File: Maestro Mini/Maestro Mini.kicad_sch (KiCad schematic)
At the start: 13 parts, among them SW1 SW_Push, SW10 SW_Push, SW2 SW_Push, SW3 SW_Push, SW4 SW_Push, SW5 SW_Push, SW6 SW_Push, SW7 SW_Push, SW8 SW_Push, SW9 SW_Push, U1 MCP23017x-x-SP

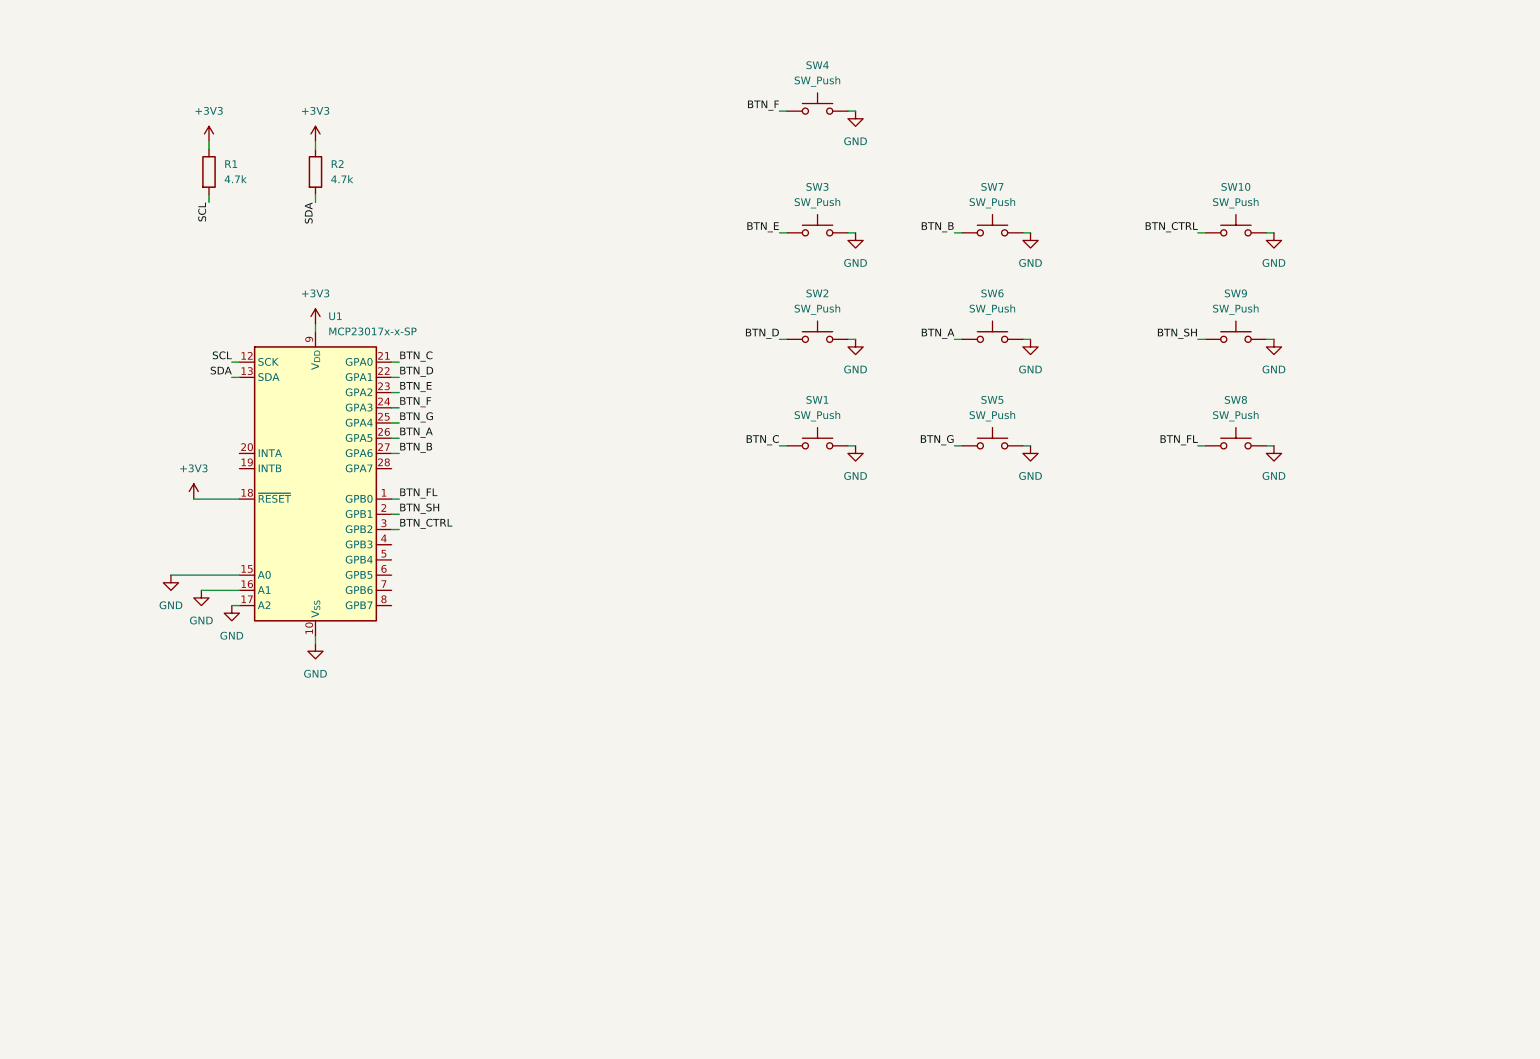
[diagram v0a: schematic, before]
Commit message: Finalized the schematics.
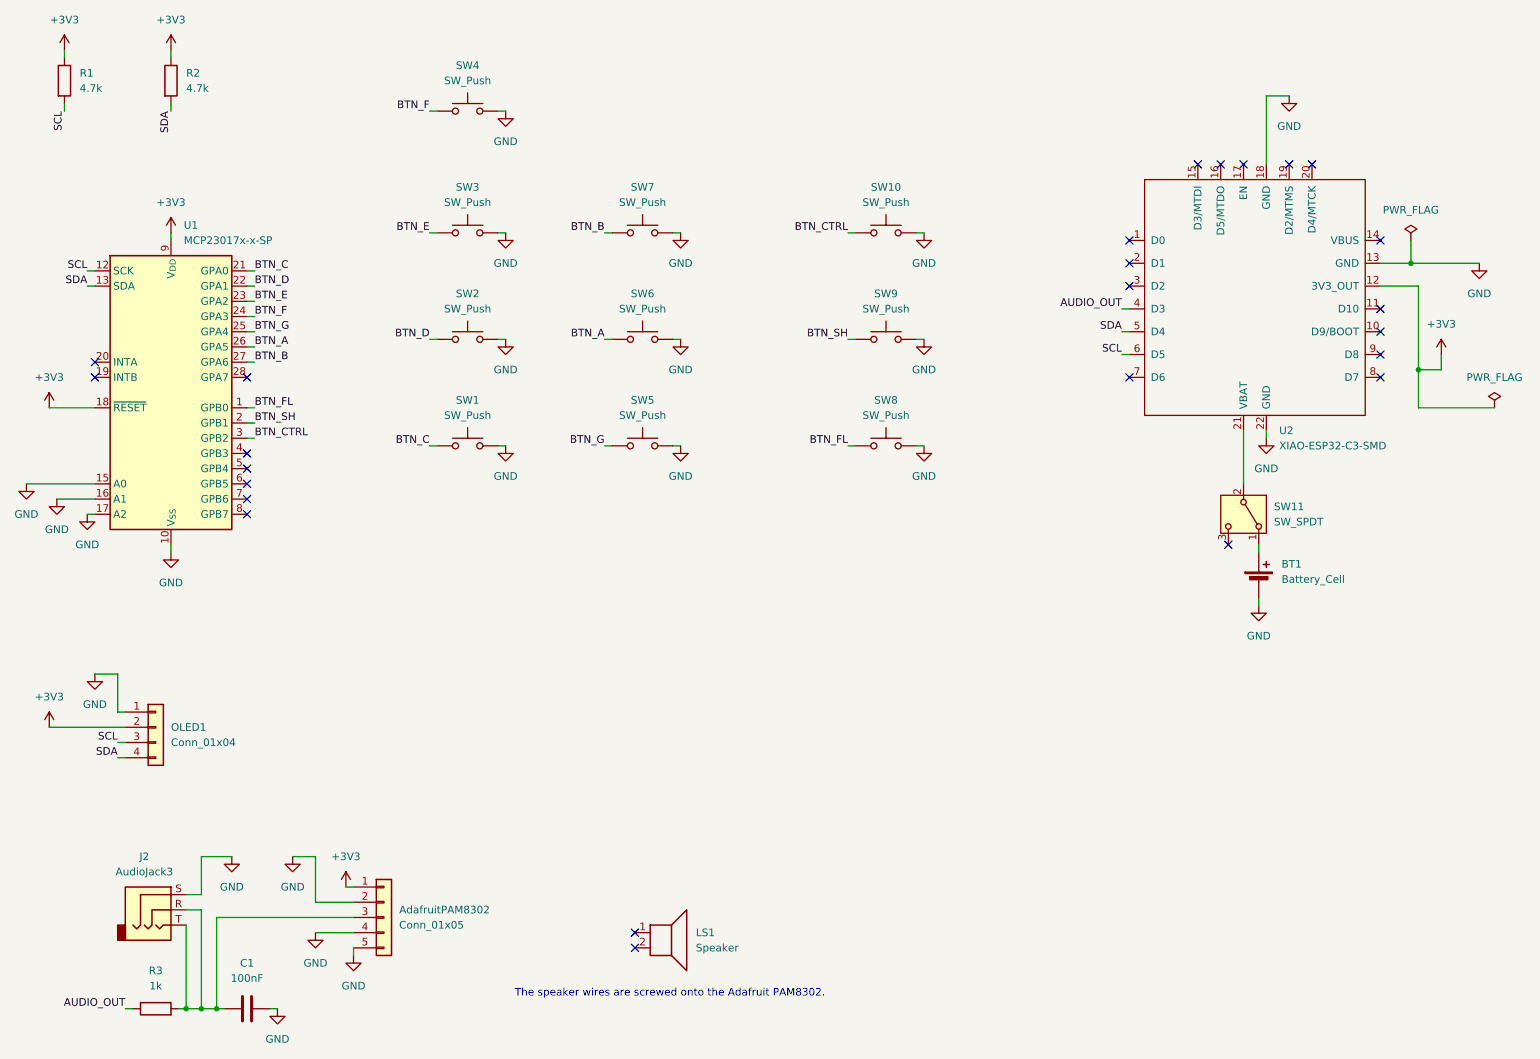
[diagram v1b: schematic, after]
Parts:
- added AdafruitPAM8302: Conn_01x05, symbol Connector_Generic:Conn_01x05
- added BT1: Battery_Cell, Package_DFN_QFN:QFN-40-1EP_6x6mm_P0.5mm_EP4.6x4.6mm, symbol Device:Battery_Cell
- added C1: 100nF, Package_SO:SOIC-8_3.9x4.9mm_P1.27mm, symbol Device:C
- added J2: AudioJack3, symbol Connector_Audio:AudioJack3
- added LS1: Speaker, symbol Device:Speaker
- added OLED1: Conn_01x04, symbol Connector_Generic:Conn_01x04
- added R3: 1k, symbol Device:R
- added SW11: SW_SPDT, symbol Switch:SW_SPDT
- added U2: XIAO-ESP32-C3-SMD, Seeed_Studio_XIAO_Series:XIAO-ESP32-C3-SMD, symbol Seeed_Studio_XIAO_Series:XIAO-ESP32-C3-SMD
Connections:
- net +3V3: now also AdafruitPAM8302.1 (Pin_1), OLED1.2 (Pin_2), U2.12 (3V3_OUT)
- net GND: now also AdafruitPAM8302.2 (Pin_2), AdafruitPAM8302.4 (Pin_4), AdafruitPAM8302.5 (Pin_5), BT1.2 (-), C1.2, J2.S, OLED1.1 (Pin_1), U2.13 (GND), U2.18 (GND), U2.22 (GND)
- net SCL: now also OLED1.3 (Pin_3), U2.6 (D5)
- net SDA: now also OLED1.4 (Pin_4), U2.5 (D4)
- new net: AdafruitPAM8302.3 (Pin_3), C1.1, J2.R, J2.T, R3.2
- new net: BT1.1 (+), SW11.1 (A)
- new net: SW11.2 (B), U2.21 (VBAT)
- new net AUDIO_OUT: R3.1, U2.4 (D3)
- no-connect marks 0 -> 25
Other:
- note added: "The speaker wires are screwed onto the Adafruit PAM8302."
- title: (none) -> Maestro Mini
- moved on the sheet: R1, R2, SW1, SW10, SW2, SW3, SW4, SW5, SW6, SW7, SW8, SW9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

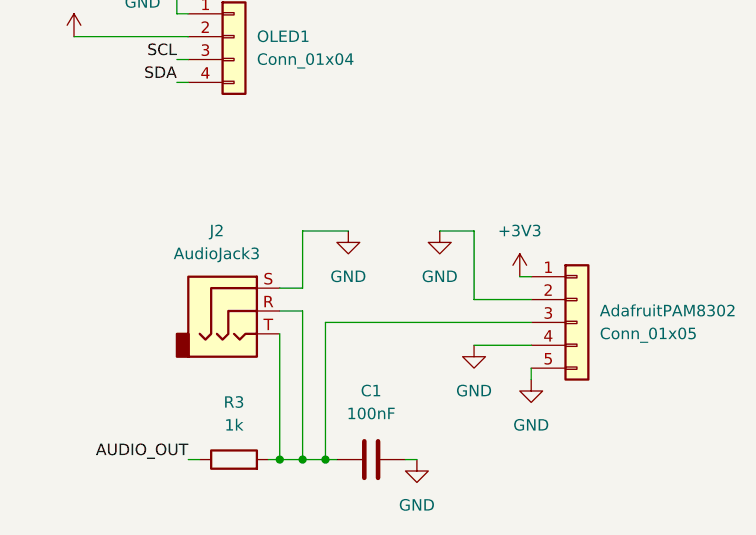
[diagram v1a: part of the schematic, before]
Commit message: Imported footprints, updated schematics, started PCB design.
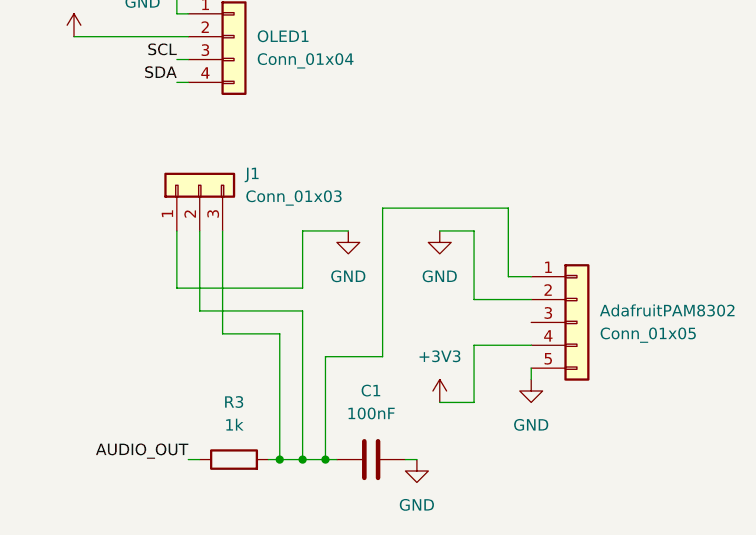
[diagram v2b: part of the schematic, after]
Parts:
- removed J2: AudioJack3, symbol Connector_Audio:AudioJack3
- added J1: Conn_01x03, Connector_PinHeader_2.54mm:PinHeader_1x03_P2.54mm_Vertical, symbol Connector_Generic:Conn_01x03
- AdafruitPAM8302: footprint (none) -> Connector_PinHeader_2.54mm:PinHeader_1x05_P2.54mm_Vertical
- BT1: footprint Package_DFN_QFN:QFN-40-1EP_6x6mm_P0.5mm_EP4.6x4.6mm -> Connector_PinHeader_2.54mm:PinHeader_1x02_P2.54mm_Vertical
- C1: footprint Package_SO:SOIC-8_3.9x4.9mm_P1.27mm -> Capacitor_THT:C_Disc_D5.0mm_W2.5mm_P5.00mm
- LS1: footprint (none) -> Connector_PinHeader_2.54mm:PinHeader_1x02_P2.54mm_Vertical
- OLED1: footprint (none) -> Imported Parts:Display_128x64_096_I2C
- R1, R2: footprint Package_DIP:DIP-28_W7.62mm -> Resistor_THT:R_Axial_DIN0204_L3.6mm_D1.6mm_P7.62mm_Horizontal
- R3: footprint (none) -> Resistor_THT:R_Axial_DIN0204_L3.6mm_D1.6mm_P7.62mm_Horizontal
- SW1, SW10, SW2, SW3, SW4, SW5, SW6, SW7, SW8, SW9: footprint Button_Switch_THT:SW_NKK_GW12LJP -> Button_Switch_Keyboard:SW_Cherry_MX_1.00u_PCB
- SW11: footprint (none) -> Connector_PinHeader_2.54mm:PinHeader_1x03_P2.54mm_Vertical
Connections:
- net +3V3: now also AdafruitPAM8302.4 (Pin_4); no longer AdafruitPAM8302.1 (Pin_1)
- net GND: now also J1.1 (Pin_1); no longer AdafruitPAM8302.4 (Pin_4)
- net at C1.1, R3.2: now also AdafruitPAM8302.1 (Pin_1), J1.2 (Pin_2), J1.3 (Pin_3); no longer AdafruitPAM8302.3 (Pin_3)
